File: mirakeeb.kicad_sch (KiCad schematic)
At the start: 148 parts, among them J1 OLED_128x64, SW1 RotaryEncoder_Switch, SW2 RotaryEncoder, U1 Raspberry_Pi_Pico

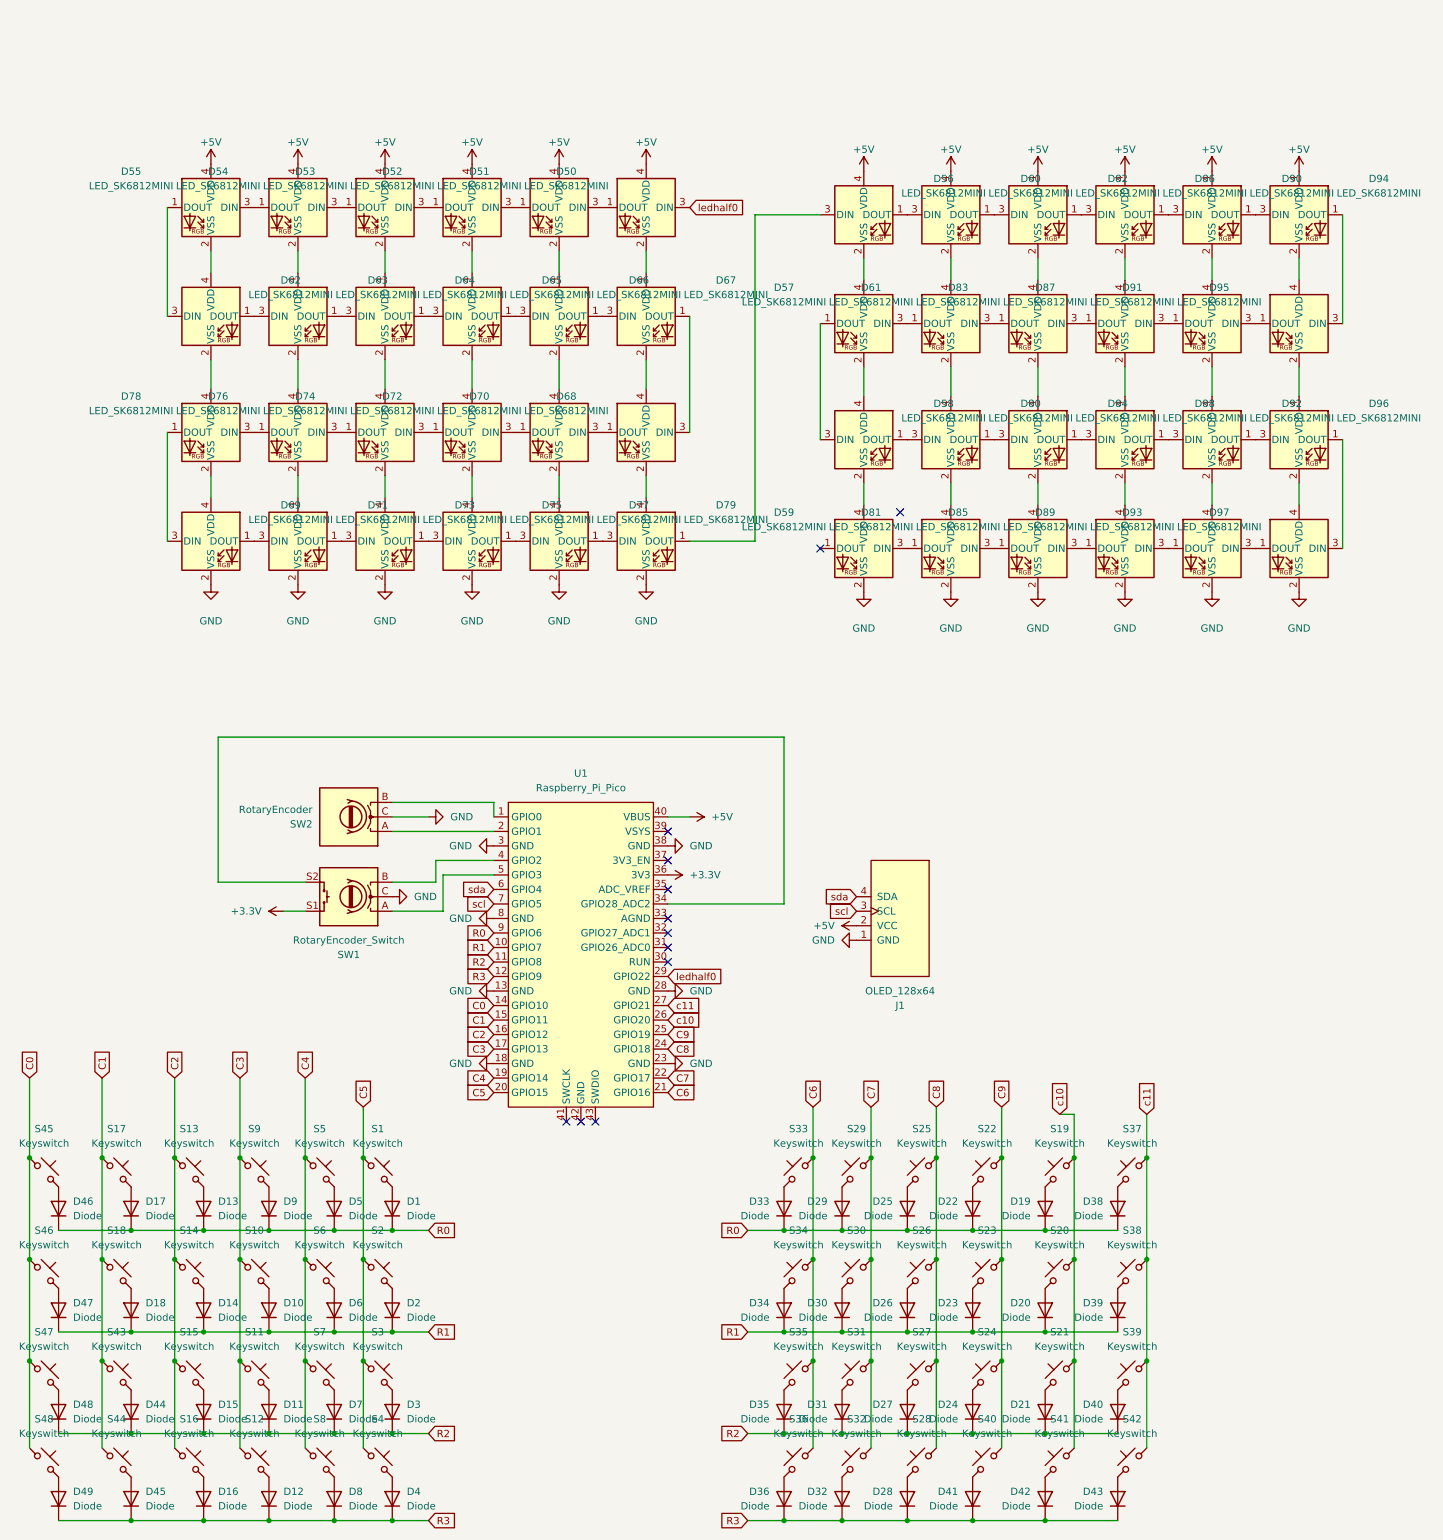
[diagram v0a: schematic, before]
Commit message: pretty much final design, just need graphics
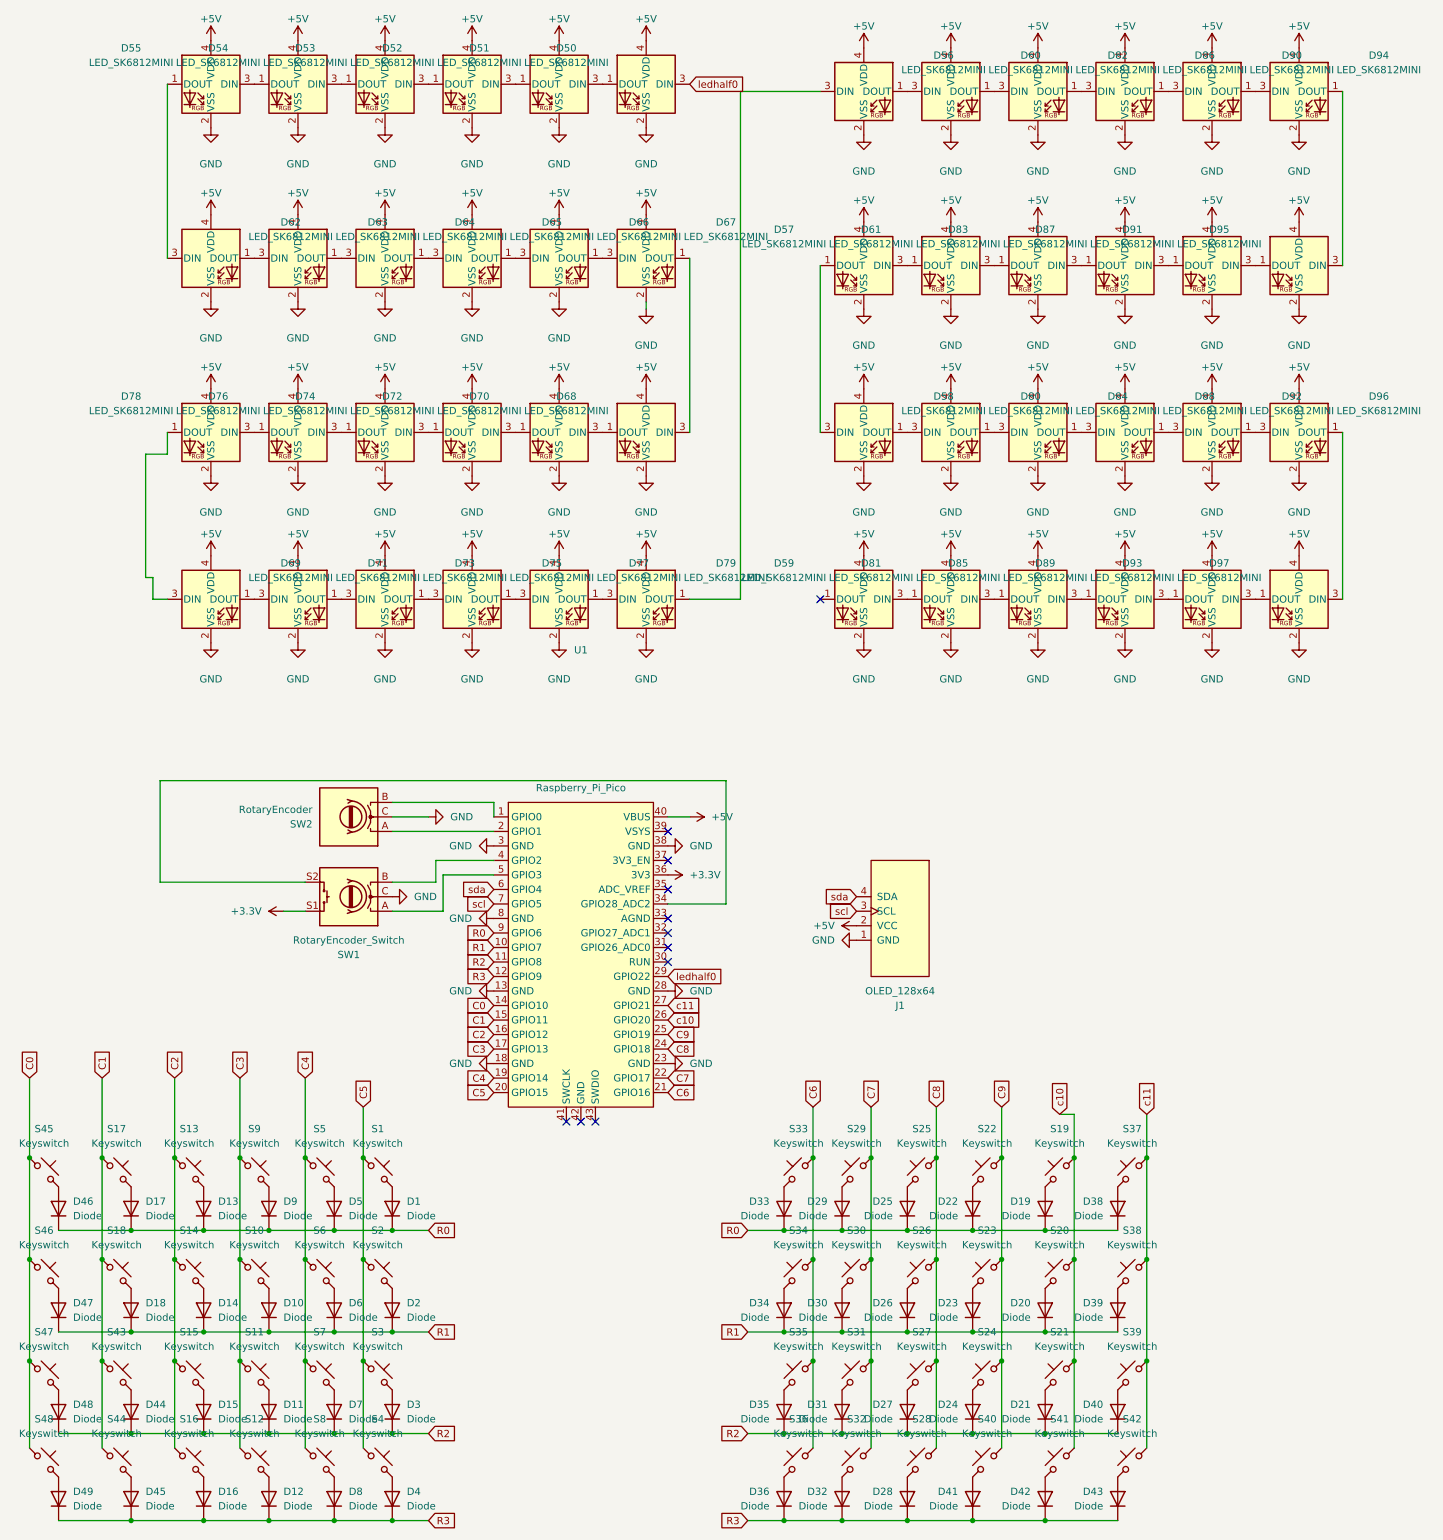
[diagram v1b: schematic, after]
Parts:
- D1, D10, D11, D12, D13, D14, D15, D16, D17, D18, D19, D2, D20, D21, D22, D23, D24, D25, D26, D27, D28, D29, D3, D30, D31, D32, D33, D34, D35, D36, D38, D39, D4, D40, D41, D42, D43, D44, D45, D46, D47, D48, D49, D5, D6, D7, D8, D9: footprint ScottoKeebs_Components:Diode_DO-35 -> scotto_components:Diode_DO-35
- D50, D51, D52, D53, D54, D55, D56, D57, D58, D59, D60, D61, D62, D63, D64, D65, D66, D67, D68, D69, D70, D71, D72, D73, D74, D75, D76, D77, D78, D79, D80, D81, D82, D83, D84, D85, D86, D87, D88, D89, D90, D91, D92, D93, D94, D95, D96, D97: footprint ScottoKeebs_Components:LED_SK6812MINI -> scotto_components:LED_SK6812MINI
- J1: footprint ScottoKeebs_Components:OLED_128x64 -> scotto_components:OLED_128x64
- S1, S10, S11, S12, S13, S14, S15, S16, S17, S18, S19, S2, S20, S21, S22, S23, S24, S25, S26, S27, S28, S29, S3, S30, S31, S32, S33, S34, S35, S36, S37, S38, S39, S4, S40, S41, S42, S43, S44, S45, S46, S47, S48, S5, S6, S7, S8, S9: footprint ScottoKeebs_MX:MX_PCB -> mx_keebs:MX_PCB_1.00u
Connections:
- net +5V: now also D57.4 (VDD), D58.4 (VDD), D59.4 (VDD), D61.4 (VDD), D62.4 (VDD), D63.4 (VDD), D64.4 (VDD), D65.4 (VDD), D66.4 (VDD), D67.4 (VDD), D68.4 (VDD), D69.4 (VDD), D70.4 (VDD), D71.4 (VDD), D72.4 (VDD), D73.4 (VDD), D74.4 (VDD), D75.4 (VDD), D76.4 (VDD), D77.4 (VDD), D78.4 (VDD), D79.4 (VDD), D80.4 (VDD), D81.4 (VDD), D83.4 (VDD), D84.4 (VDD), D85.4 (VDD), D87.4 (VDD), D88.4 (VDD), D89.4 (VDD), D91.4 (VDD), D92.4 (VDD), D93.4 (VDD), D95.4 (VDD), D96.4 (VDD), D97.4 (VDD)
- net GND: now also D50.2 (VSS), D51.2 (VSS), D52.2 (VSS), D53.2 (VSS), D54.2 (VSS), D55.2 (VSS), D56.2 (VSS), D57.2 (VSS), D58.2 (VSS), D60.2 (VSS), D61.2 (VSS), D62.2 (VSS), D63.2 (VSS), D64.2 (VSS), D65.2 (VSS), D66.2 (VSS), D67.2 (VSS), D68.2 (VSS), D70.2 (VSS), D72.2 (VSS), D74.2 (VSS), D76.2 (VSS), D78.2 (VSS), D80.2 (VSS), D82.2 (VSS), D83.2 (VSS), D84.2 (VSS), D86.2 (VSS), D87.2 (VSS), D88.2 (VSS), D90.2 (VSS), D91.2 (VSS), D92.2 (VSS), D94.2 (VSS), D95.2 (VSS), D96.2 (VSS)
- no-connect marks 12 -> 11
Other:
- moved on the sheet: D50, D51, D52, D53, D54, D55, D56, D57, D58, D59, D60, D61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
